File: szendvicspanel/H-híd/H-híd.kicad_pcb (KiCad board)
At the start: 2 copper layers, 29.5 x 39 mm, 12 parts, among them J1 Conn_01x03_Pin, J2 Conn_01x02_Socket, Q1 BS170, Q2 BS170, Q3 BS170, Q4 BS170, Q5 BS250, Q6 BS250

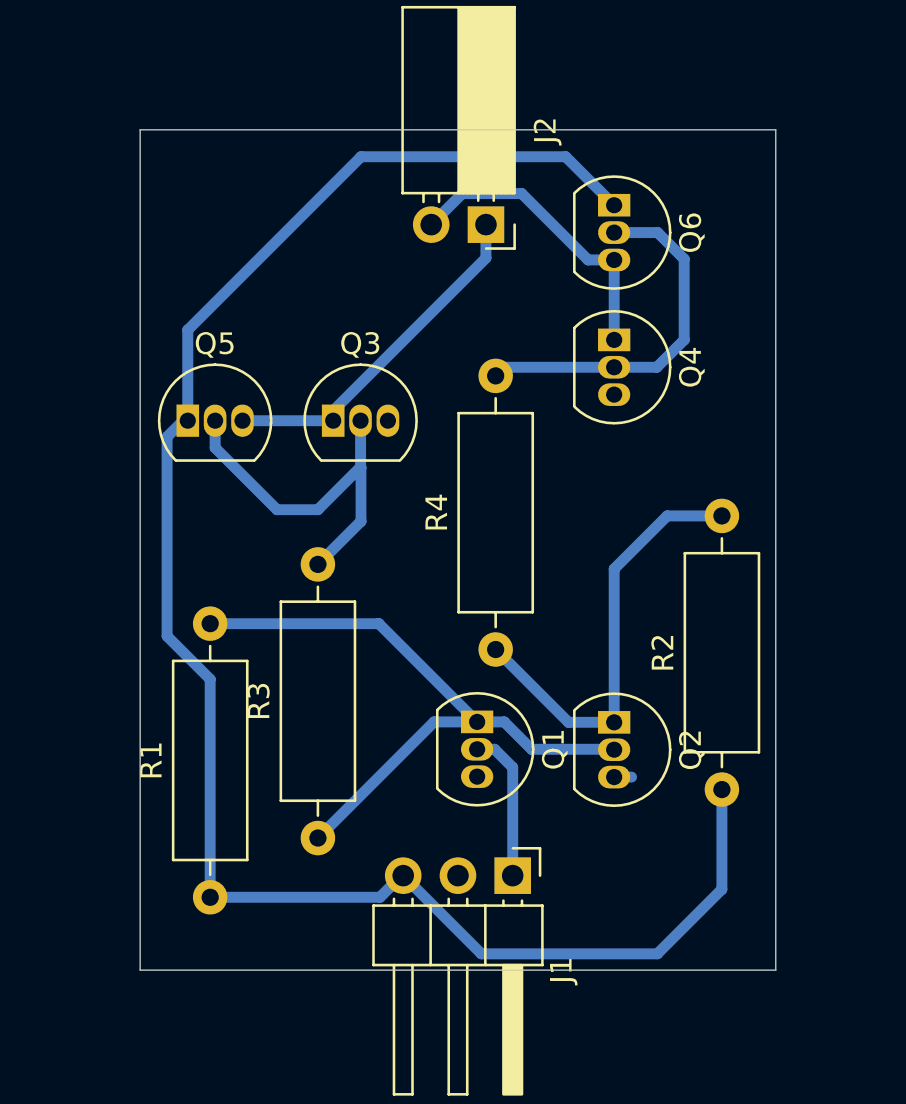
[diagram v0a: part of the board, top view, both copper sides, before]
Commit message: A H-hidat picit átdizájnoltam
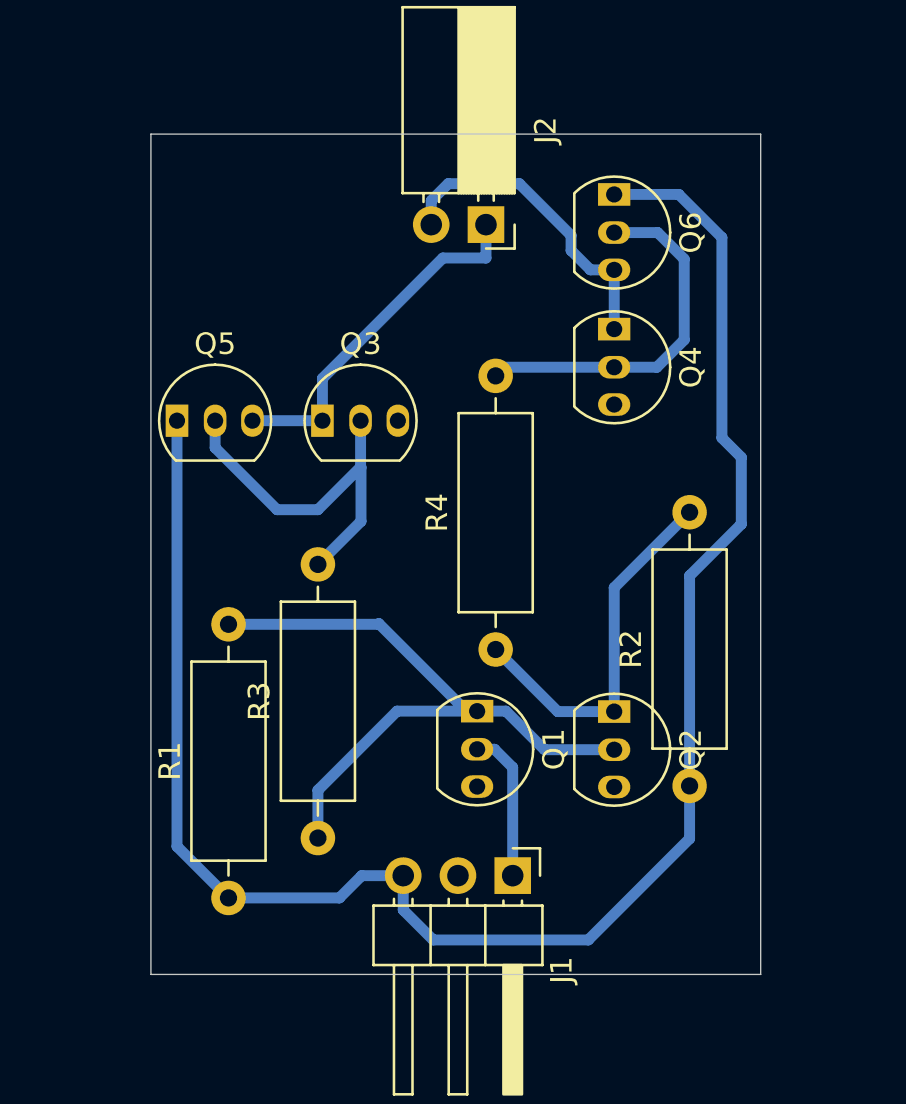
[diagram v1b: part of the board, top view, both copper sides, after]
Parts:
- moved R2 1.51 mm to (236.5, 115.0)
- moved R1 0.85 mm to (215.1, 120.2)
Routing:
- net Net-(Q2-D): track 20.0 -> 17.4 mm
- net /VPWR: track 83.4 -> 84.3 mm
- net GND: track 0.81 -> 0.00 mm
- net Net-(Q1-D): track 30.8 -> 31.5 mm
- net /OUT_B: track 14.1 -> 14.7 mm
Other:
- board size 29.5 x 39 mm -> 28.3 x 39 mm
